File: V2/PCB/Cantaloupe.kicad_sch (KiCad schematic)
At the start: 121 parts, among them J1 USB_In, J2 OLED, J3 Link, J4 Debug, J5 Trackball, Q1 2N7002, Q2 AO3401A, SW1 MX, SW10 MX, SW11 MX, SW12 MX, SW13 MX, SW14 MX, SW15 MX, SW16 MX, SW17 MX, SW18 MX, SW19 MX, SW2 MX, SW20 MX, SW21 MX, SW22 MX, SW23 MX, SW24 MX, SW25 MX, SW26 MX, SW27 MX, SW28 MX, SW29 MX, SW3 MX, SW30 MX, SW31 Encoder, SW32 MX, SW4 MX, SW5 MX, SW6 MX, SW7 MX, SW8 MX, SW9 MX, U1 STM32F4x1CxUx, U2 SRV0504, U3 SRV0504, U4 XC6206P332MR, U5 LMV321, Y1 8MHz

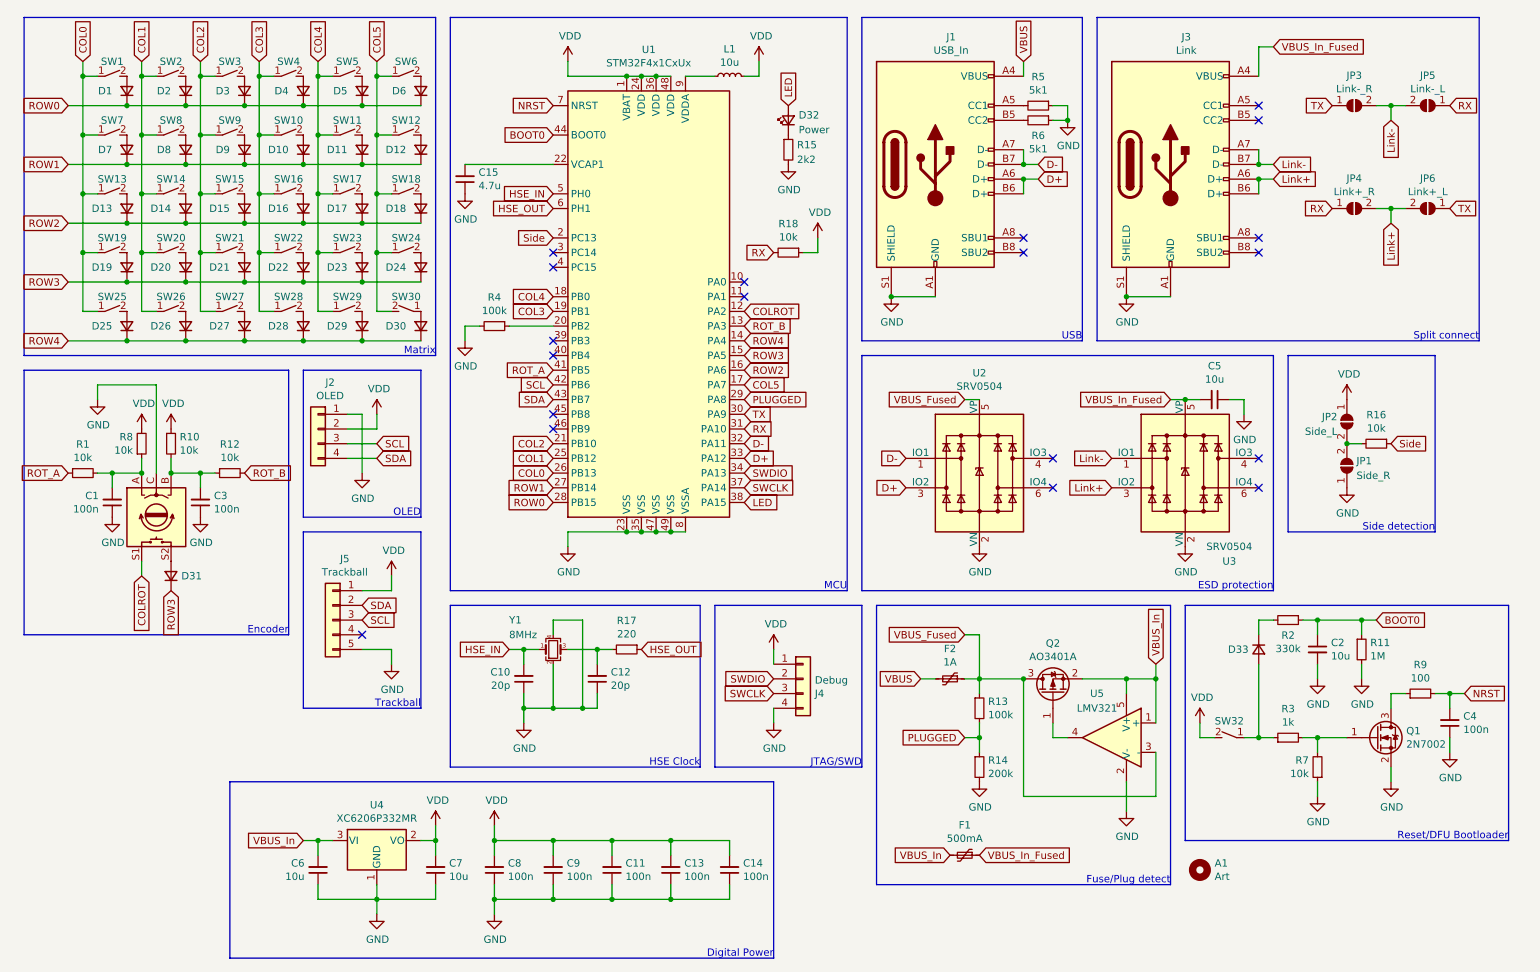
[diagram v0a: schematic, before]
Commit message: Tentative V2.1 update
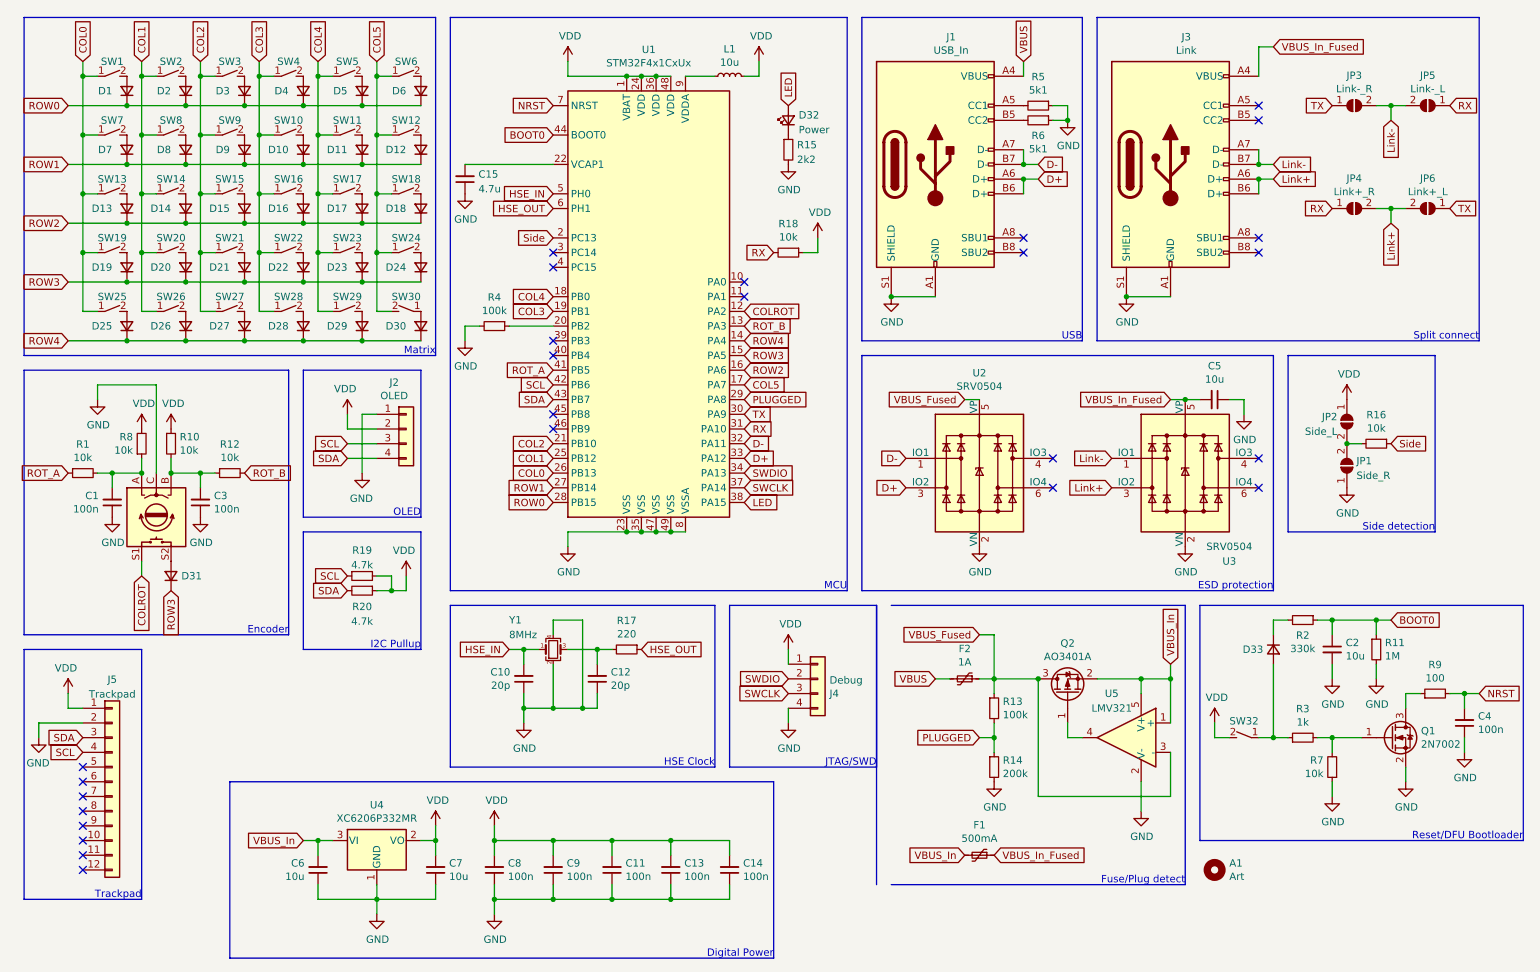
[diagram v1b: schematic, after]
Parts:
- removed J5: Trackball, Ariamelon:pimoroni_trackball_flippable, symbol Connector_Generic:Conn_01x05
- added J5: Trackpad, Ariamelon:FPC-SMD_FPC05012-09200-.5mm-rev, symbol Connector_Generic:Conn_01x12
- added R19, R20: 4.7k, Resistor_SMD:R_0603_1608Metric, symbol Device:R_Small
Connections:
- net GND: now also J5.2 (Pin_2)
- net SCL: now also J5.4 (Pin_4), R19.1
- net SDA: now also J5.3 (Pin_3), R20.2
- net VDD: now also J5.1 (Pin_1), R19.2, R20.1
- no-connect marks 19 -> 26
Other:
- note added: "I2C Pullup"
- note added: "Trackpad"
- note removed: "Trackball"
- moved on the sheet: A1, C2, C4, D33, F1, F2, J2, J4, Q1, Q2, R11, R13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
